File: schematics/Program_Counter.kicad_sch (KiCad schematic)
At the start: 19 parts, among them U1 74LS173, U2 74LS173

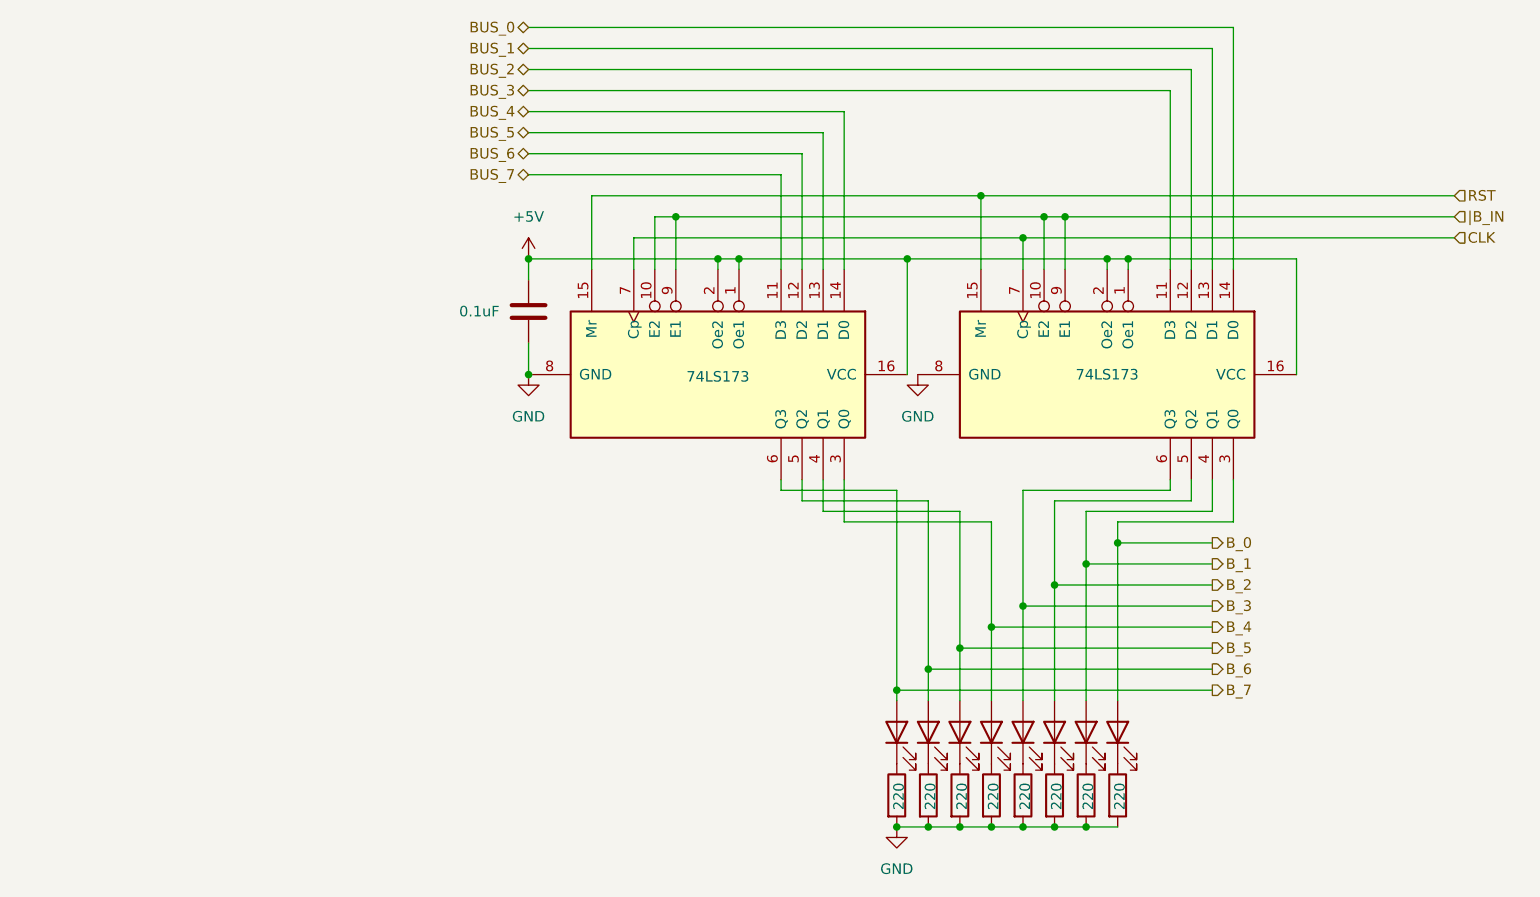
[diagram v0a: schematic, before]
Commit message: chore: more docs and schematics
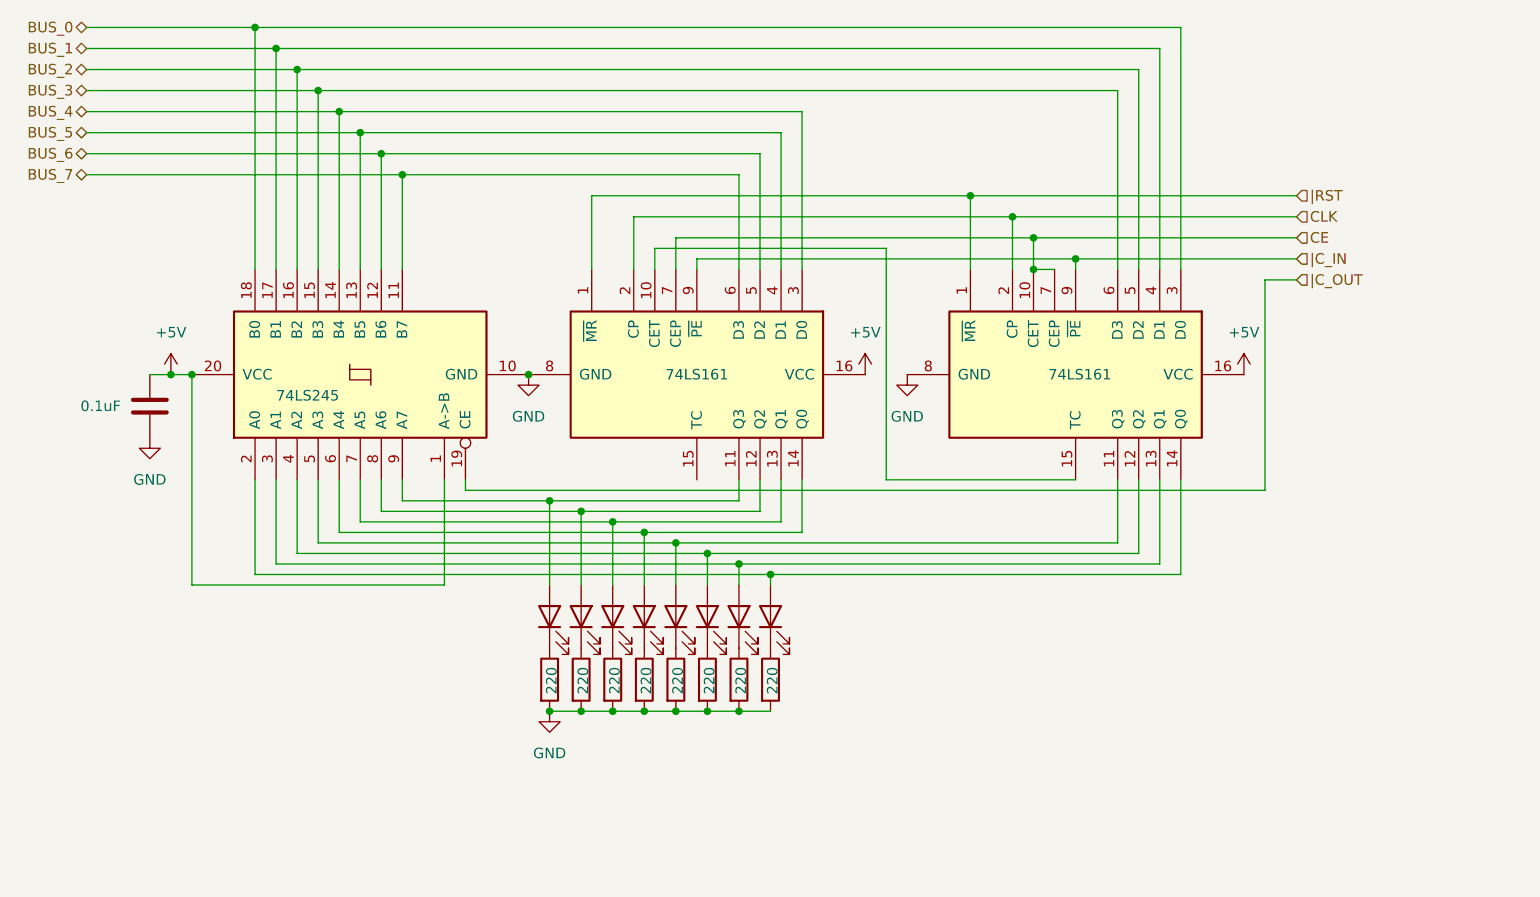
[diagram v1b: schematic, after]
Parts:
- removed U1, U2: 74LS173, symbol 74xx:74LS173
- added U1, U2: 74LS161, symbol 74xx:74LS161
- added U3: 74LS245, symbol 74xx:74LS245
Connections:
- net +5V: now also U1.16 (VCC), U2.16 (VCC), U3.1 (A->B), U3.20 (VCC)
- net BUS_0: now also U2.3 (D0), U3.18 (B0)
- net BUS_1: now also U2.4 (D1), U3.17 (B1)
- net BUS_2: now also U2.5 (D2), U3.16 (B2)
- net BUS_3: now also U2.6 (D3), U3.15 (B3)
- net BUS_4: now also U1.3 (D0), U3.14 (B4)
- net BUS_5: now also U1.4 (D1), U3.13 (B5)
- net BUS_6: now also U1.5 (D2), U3.12 (B6)
- net BUS_7: now also U1.6 (D3), U3.11 (B7)
- net CLK: now also U1.2 (CP), U2.2 (CP)
- net GND: now also U1.8 (GND), U2.8 (GND), U3.10 (GND)
- net B_0: no longer names the net of D8.2 (A)
- net B_0: now also U2.14 (Q0), U3.2 (A0)
- net B_1: no longer names the net of D7.2 (A)
- net B_1: now also U2.13 (Q1), U3.3 (A1)
- net B_2: no longer names the net of D6.2 (A)
- net B_2: now also U2.12 (Q2), U3.4 (A2)
- net B_3: no longer names the net of D5.2 (A)
- net B_3: now also U2.11 (Q3), U3.5 (A3)
- net B_4: no longer names the net of D4.2 (A)
- net B_4: now also U1.14 (Q0), U3.6 (A4)
- net B_5: no longer names the net of D3.2 (A)
- net B_5: now also U1.13 (Q1), U3.7 (A5)
- net B_6: no longer names the net of D2.2 (A)
- net B_6: now also U1.12 (Q2), U3.8 (A6)
- net B_7: no longer names the net of D1.2 (A)
- net B_7: now also U1.11 (Q3), U3.9 (A7)
- new net: U1.10 (CET), U2.15 (TC)
- new net CE: U1.7 (CEP), U2.10 (CET), U2.7 (CEP)
- new net |C_IN: U1.9 (~{PE}), U2.9 (~{PE})
- new net |C_OUT: U3.19 (CE)
- new net |RST: U1.1 (~{MR}), U2.1 (~{MR})
